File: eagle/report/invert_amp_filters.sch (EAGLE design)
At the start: 7 parts, among them IC1 LM324N

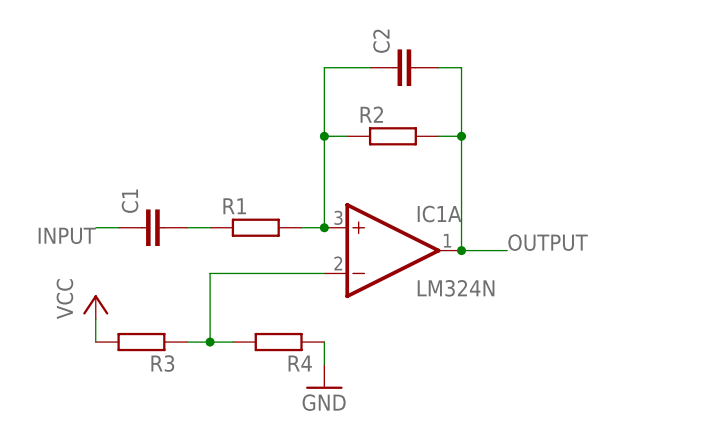
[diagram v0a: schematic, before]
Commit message: Continued design and implementation.
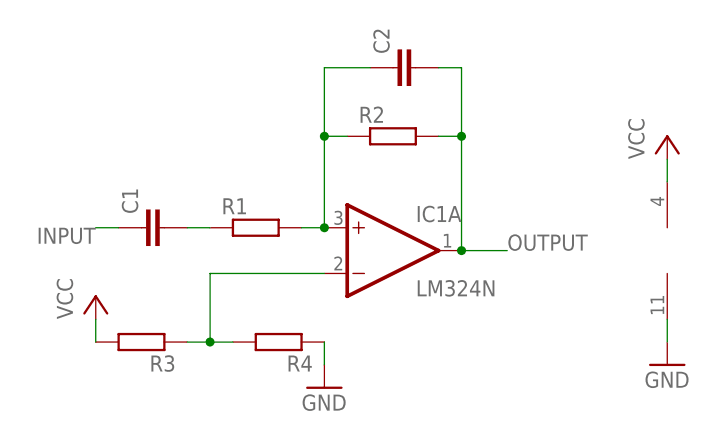
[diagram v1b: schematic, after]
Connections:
- net GND: now also IC1P.V-
- net VCC: now also IC1P.V+
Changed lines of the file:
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@@
 <?xml version="1.0" encoding="utf-8"?>
 <!DOCTYPE eagle SYSTEM "eagle.dtd">
-<eagle version="6.3">
+<eagle version="6.4">
 <drawing>
 <settings>
@@
 <part name="P+1" library="supply1" deviceset="VCC" device=""/>
 <part name="GND1" library="supply1" deviceset="GND" device=""/>
+<part name="P+2" library="supply1" deviceset="VCC" device=""/>
+<part name="GND2" library="supply1" deviceset="GND" device=""/>
 </parts>
 <sheets>
@@
 <instance part="P+1" gate="VCC" x="27.94" y="43.18"/>
 <instance part="GND1" gate="1" x="53.34" y="33.02"/>
+<instance part="IC1" gate="P" x="91.44" y="48.26"/>
+<instance part="P+2" gate="VCC" x="91.44" y="60.96"/>
+<instance part="GND2" gate="1" x="91.44" y="35.56"/>
 </instances>
 <busses>
@@
 <wire x1="27.94" y1="40.64" x2="27.94" y2="38.1" width="0.1524" layer="91"/>
 </segment>
+<segment>
+<pinref part="IC1" gate="P" pin="V+"/>
+<pinref part="P+2" gate="VCC" pin="VCC"/>
+<wire x1="91.44" y1="58.42" x2="91.44" y2="55.88" width="0.1524" layer="91"/>
+</segment>
 </net>
 <net name="GND" class="0">
@@
 <wire x1="53.34" y1="35.56" x2="53.34" y2="38.1" width="0.1524" layer="91"/>
 </segment>
+<segment>
+<pinref part="IC1" gate="P" pin="V-"/>
+<pinref part="GND2" gate="1" pin="GND"/>
+<wire x1="91.44" y1="38.1" x2="91.44" y2="40.64" width="0.1524" layer="91"/>
+</segment>
 </net>
